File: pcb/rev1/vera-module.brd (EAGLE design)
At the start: 57 x 75 mm, 75 parts, among them J1 ICD15S13E4GX00LF, J2 RCJ-014, J3 HDR8X1, J4 C64CART, J5 BUS, Q1 BC847SOT-23, U1 ICE40UP5K-SG48ITR50, U2 MIC5504-3.3YM5-TR, U3 SN74CBTD3861PWR, U4 W25Q16JVSNIQ, U5 SG5032CAN_25.000000M-TJGA3, U6 74LVC4245APW, U8 AP3417CKTR-G1, U9 74AHCT1G14SE-7

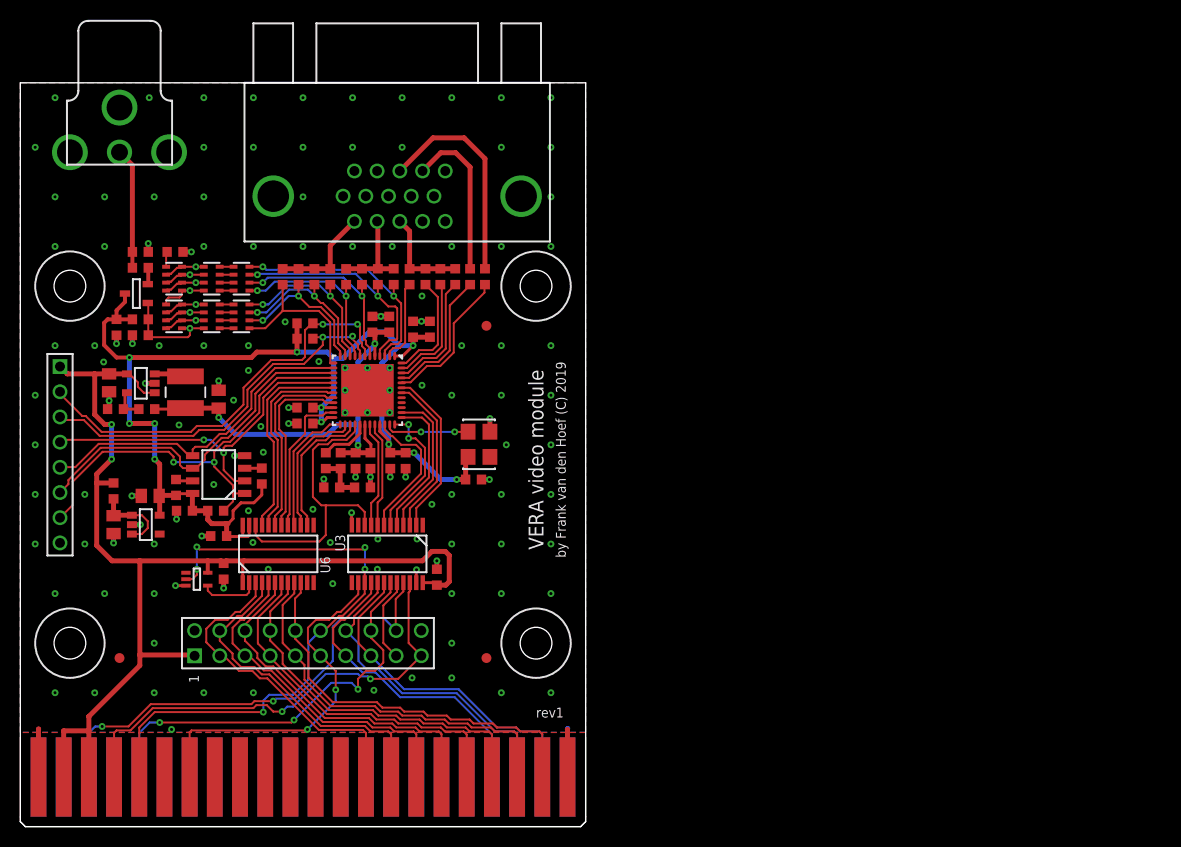
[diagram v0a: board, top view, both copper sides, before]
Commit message: Finished work on rev1 VERA PCB.
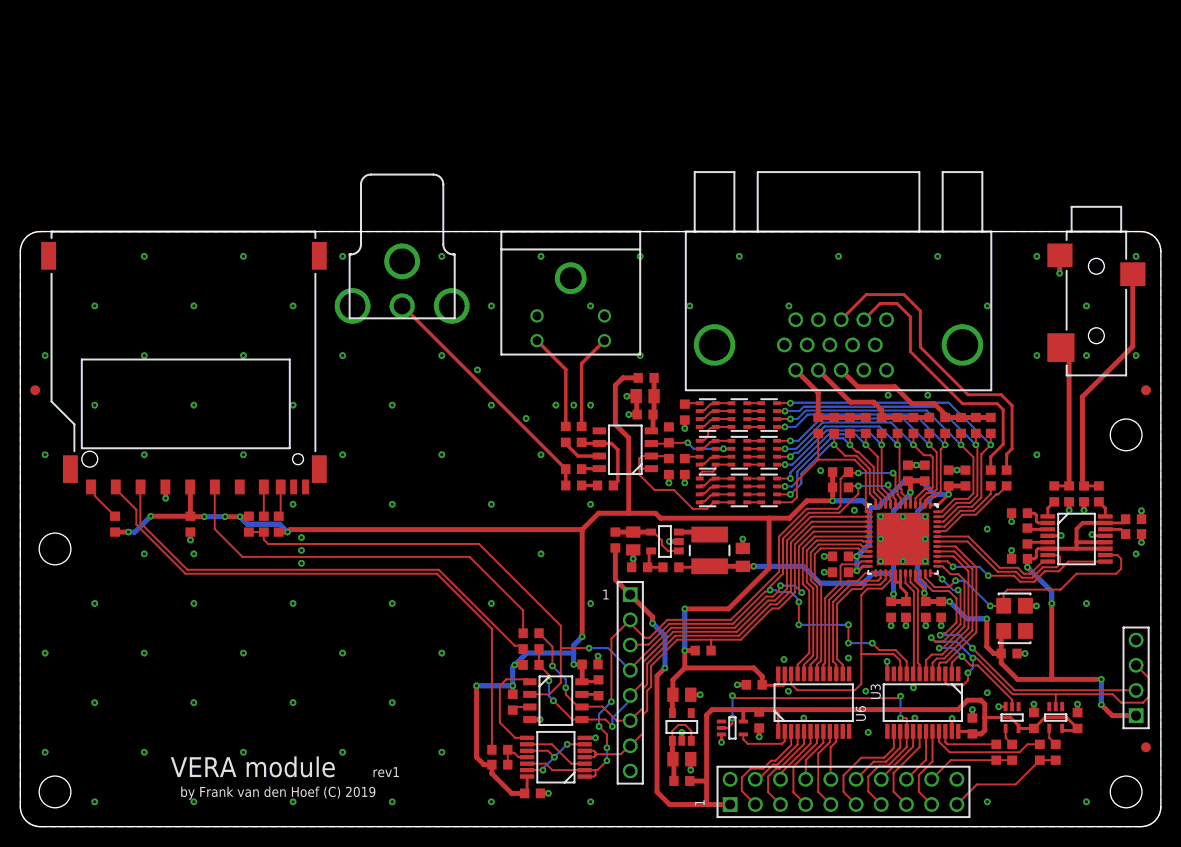
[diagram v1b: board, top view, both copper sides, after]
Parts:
- removed Q1: BC847SOT-23, transistor:SOT-23-3
- added C20, C21: 1u, rcl:C0603
- added C22, C24, C28: 4.7u, rcl:C0603
- added C27: 2.2u, rcl:C0603
- added C29, C30, C31: 100n, rcl:C0603
- added C3: 1n, rcl:C0603
- added J6: AUDIO, connectors:35RASMT2BHNTRX
- added J7: 2041021-3, connectors:2041021-3
- added J9: SERIAL, connectors:HDR4X1
- added R23: 470, rcl:R0603
- added R24: 1k, rcl:R0603
- added R29, R30, R31: CAY16-1001F4LF, rcl:RA4_1206
- added R32: 75, rcl:R0603
- added R33, R36, R50, R52: 0, rcl:R0603
- added R37: 1, rcl:R0603
- added R38, R39: 560, rcl:R0603
- added R42, R47, R48: 47k, rcl:R0603
- added R49, R51: DNP, rcl:R0603
- added R53, R54, R55, R56: 100, rcl:R0603
- added U10: WM8524CGEDT, integrated_circuits:TSSOP-16
- added U11: 74AHC00PW, integrated_circuits:TSSOP-14
- added U12, U13: 74AHCT1G14SE-7, integrated_circuits:TSSOP-5
- added U7: THS7314D, integrated_circuits:SOIC-8
- C1: value 22p -> 100n
- C16: value 100n -> 2.7n
- C17: value 4.7u -> 2.7n
- C2: value 100n -> 10u; device rcl:C0603 -> rcl:C0805
- J4: value C64CART -> MD-40S; device connectors:C64CART -> connectors:MD-40S
- R25: value 1k -> 470
- R26, R27: value 1k -> 75
- R40: value 100 -> 47k
- R41: value 1 -> 47k
- moved C17 74.4 mm to (105.8, 33.5), turned to 90 degrees
- moved C16 72.8 mm to (107.2, 33.5), turned to 90 degrees
- moved FD2 67.1 mm to (113.5, 8.00)
- moved FD3 66.8 mm to (113.5, 44.0)
- moved J4 65.8 mm to (55.5, 60.0)
- moved R28 64.3 mm to (66.7, 4.60), turned to 180 degrees
- moved C69 62.0 mm to (66.7, 6.80), turned to 180 degrees
- moved J3 61.9 mm to (61.5, 14.5)
- moved U2 57.8 mm to (66.7, 10.1), turned to 90 degrees
- moved C70 57.2 mm to (66.7, 13.3), turned to 180 degrees
- moved C18 56.8 mm to (99.7, 17.4)
- moved U5 56.8 mm to (100.2, 21.0)
- moved R14 56.6 mm to (69.3, 33.9)
- moved R15 56.6 mm to (69.3, 37.7)
- moved R5 56.4 mm to (99.5, 35.1)
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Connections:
- removed net BUS_RES#: U1.42, U3.3
- removed net COMPOSITE: J2.S, R26.1, R27.2
- new net AUDIO_BCK: U1.38, U10.9
- new net AUDIO_DATA: U1.42, U10.7
- new net AUDIO_LRCK: U1.43, U10.8
- new net BUS_PHY2_5V_IN: R50.1, U3.22
- new net BUS_RDY_5V_OD: R52.1, U3.21
- new net FLASH_SSEL_N: U11.8, U4.1
- new net N$23: R32.1, U7.8
- new net N$24: C3.1, R33.2
- new net N$27: R29.2A, R30.2B
- new net N$28: R29.3A, R30.3B
- new net N$30: R29.4A, R30.4B
- new net N$31: R15.4A, R30.1A, R31.1B
- new net N$32: R30.2A, R31.1A, R31.2B
- new net N$33: R30.3A, R31.2A, R31.3B
- new net N$34: R24.1, R31.4A
- new net N$35: R30.4A, R31.3A, R31.4B
- new net N$36: R26.1, U7.7
- new net N$37: C1.2, C2.2, R36.1, U7.4
- new net N$38: C17.2, J6.4, R38.2
- new net N$39: C16.2, J6.1, R39.2
- new net N$40: R38.1, U10.1
- new net N$41: R39.1, U10.16
- new net N$42: C20.1, U10.5
- new net N$43: J7.8, R47.2
- new net N$45: C21.2, U10.2
- new net N$46: U11.3, U11.9
- new net N$47: U11.10, U11.13, U11.6
- new net N$48: R49.1, U12.4
- new net N$49: C27.2, U10.14
- new net N$50: R51.1, U13.4
- new net N$51: J7.2, R54.2
- new net N$52: J7.5, R53.2
- new net N$53: J7.1, R56.2
- new net N$54: J7.7, R55.2
- new net SD_SSEL_N: R40.2, R56.1, U11.11
- new net UART_RX: J9.2, U1.34
- new net VIDEO_C: J4.4, R27.2
- new net VIDEO_CHROMA: R15.3B, R25.2, R7.3A, U7.3
- new net VIDEO_COMP: C3.2, J2.S, R32.2
- new net VIDEO_LUMA: R14.1B, R23.2, R3.1A, U7.1, U7.2
- new net VIDEO_Y: J4.3, R26.2
- net +1.2V: now also U1.29; no longer R41.2
- net +3.3V: now also C22.2, C24.2, C28.1, C29.2, J7.4, J9.1, R36.2, R40.1, R41.1, R42.1, R47.1, R48.1, U10.11, U10.12, U10.15, U10.6, U11.14; no longer C2.1, Q1.3, R25.2
- net +5V: now also C30.2, C31.2, R37.1, U12.5, U13.5; no longer C25.2, J4.2, J4.3, U8.1, U8.4
- net BUS_A0: now also U1.41, U3.4; no longer U1.36, U3.6
- net BUS_A0_5V: now also J5.17, U3.20; no longer J4.Y, J5.15, U3.18
- net BUS_A1: now also U1.40, U3.5; no longer U1.34, U3.7
- net BUS_A1_5V: now also J5.16, U3.19; no longer J4.X, J5.14, U3.17
- net BUS_A2: now also U1.39, U3.6; no longer U1.32, U3.8
- net BUS_A2_5V: now also J5.15, U3.18; no longer J4.W, J5.13, U3.16
- net BUS_CS#_5V: no longer J4.7
- net BUS_D0_5V: no longer J4.21
- net BUS_D1_5V: no longer J4.20
- net BUS_D2_5V: no longer J4.19
- net BUS_D3_5V: no longer J4.18
- net BUS_D4_5V: no longer J4.17
- net BUS_D5_5V: no longer J4.16
- net BUS_D6_5V: no longer J4.15
- net BUS_D7_5V: no longer J4.14
- net BUS_IRQ#: now also U1.32, U3.7; no longer U1.43, U3.2
- net BUS_IRQ#_5V: now also J5.14, U3.17; no longer J4.4, J5.19, U3.22
- net BUS_PHY2: now also U12.2, U3.2; no longer U3.5
- net BUS_PHY2_5V: now also J5.18, R49.2, R50.2; no longer J4.E, J5.16, U3.19
- net BUS_RDY: now also J9.3, U1.36, U13.2, U3.3; no longer U1.38, U3.4
- net BUS_RDY_5V: now also J5.19, R51.2, R52.2; no longer J5.17, U3.20
- net BUS_RES#_5V: now also J5.12, U3.15; no longer J4.C, J5.18, U3.21
- net BUS_RW#: now also U3.8; no longer U3.9
- net BUS_RW#_5V: now also J5.13, U3.16; no longer J4.5, J5.12, U3.15
- net FPGA_CDONE: now also U11.1, U11.12, U11.2
- net FPGA_CRESET_B: now also U3.9
- net GND: now also C2.1, C21.1, C22.1, C24.1, C27.1, C28.2, C29.1, C30.1, C31.1, J1.MH1, J1.MH2, J4.2, J4.MH, J6.5, J7.3, J7.6, J7.MP1, J7.MP2, J7.MP3, J7.MP4, J9.4, R23.1, R24.2, R25.1, U10.13, U10.4, U11.7, U12.3, U13.3, U7.5; no longer C2.2, J4.22, J4.A, J4.Z, R27.1
- net N$12: now also R27.1, R33.1, U7.6; no longer C1.2, Q1.1, R14.1B, R25.1, R3.1A
- net N$22: now also C25.2, R37.2, U8.1, U8.4; no longer R15.2A, R15.3B, R7.3A
- net N$26: now also C20.2, U10.3; no longer Q1.2, R26.2
- net N$29: now also R15.2A; no longer R15.4A
- net N$44: now also J7.9, R48.2; no longer R40.1, U1.29
- net N$9: now also R29.1A, R30.1B; no longer C16.2, C17.2, R40.2, R41.1
- net SPI_MISO: now also R42.2, R55.1
- net SPI_MOSI: now also R41.2, R54.1
- net SPI_SCK: now also R53.1
- net SPI_SSEL_N: now also U11.4, U11.5; no longer U4.1
- net SYSCLK: now also U10.10
- net VGA_B0: now also R29.4B
- net VGA_B1: now also R29.3B
- net VGA_B2: now also R29.2B
- net VGA_B3: now also R29.1B
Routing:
- net +3.3V: track 127.0 -> 296.3 mm, vias 11 -> 24
- net N$53: track 0.00 -> 57.1 mm
- net SPI_MISO: track 36.7 -> 87.0 mm, vias 2 -> 3
- net N$51: track 0.00 -> 47.5 mm
- net BUS_IRQ#_5V: track 47.6 -> 6.16 mm, vias 2 -> 0
- net N$52: track 0.00 -> 41.1 mm
- net BUS_RES#_5V: track 48.0 -> 7.41 mm, vias 2 -> 0
- net BUS_D0_5V: track 40.7 -> 5.08 mm
- net BUS_PHY2_5V: track 42.5 -> 8.91 mm, vias 3 -> 0
- net BUS_D2_5V: track 37.8 -> 5.57 mm
- net UART_RX: track 0.00 -> 31.7 mm, vias 0 -> 2
- net BUS_RDY: track 15.1 -> 46.7 mm, vias 0 -> 5
- net BUS_D1_5V: track 39.2 -> 8.39 mm
- net BUS_D4_5V: track 35.4 -> 6.08 mm
- net BUS_A1_5V: track 33.2 -> 5.65 mm
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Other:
- board size 57 x 75 mm -> 115 x 60 mm
- board text added: "5V"
- board text added: "A0"
- board text added: "A1"
- board text added: "A2"
- board text added: "CS#"
- board text added: "D0"
- board text added: "D1"
- board text added: "D2"
- board text added: "D3"
- board text added: "D4"
- board text added: "D5"
- board text added: "D6"
- board text added: "D7"
- board text added: "GND"
- board text added: "IRQ#"
- board text added: "PHY2"
- board text added: "RDY"
- board text added: "RES#"
- board text added: "RW#"
- board text added: "VERA module"
- board text removed: "VERA video module"
